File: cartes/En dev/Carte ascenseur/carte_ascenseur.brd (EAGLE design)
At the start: 96.5 x 93.9 mm, 35 parts, among them U1 MCP2551, U2 ADUM1250ARZ, U3 ADUM1400ARWZ, X1 12V Dirty, X2 5V Dirty

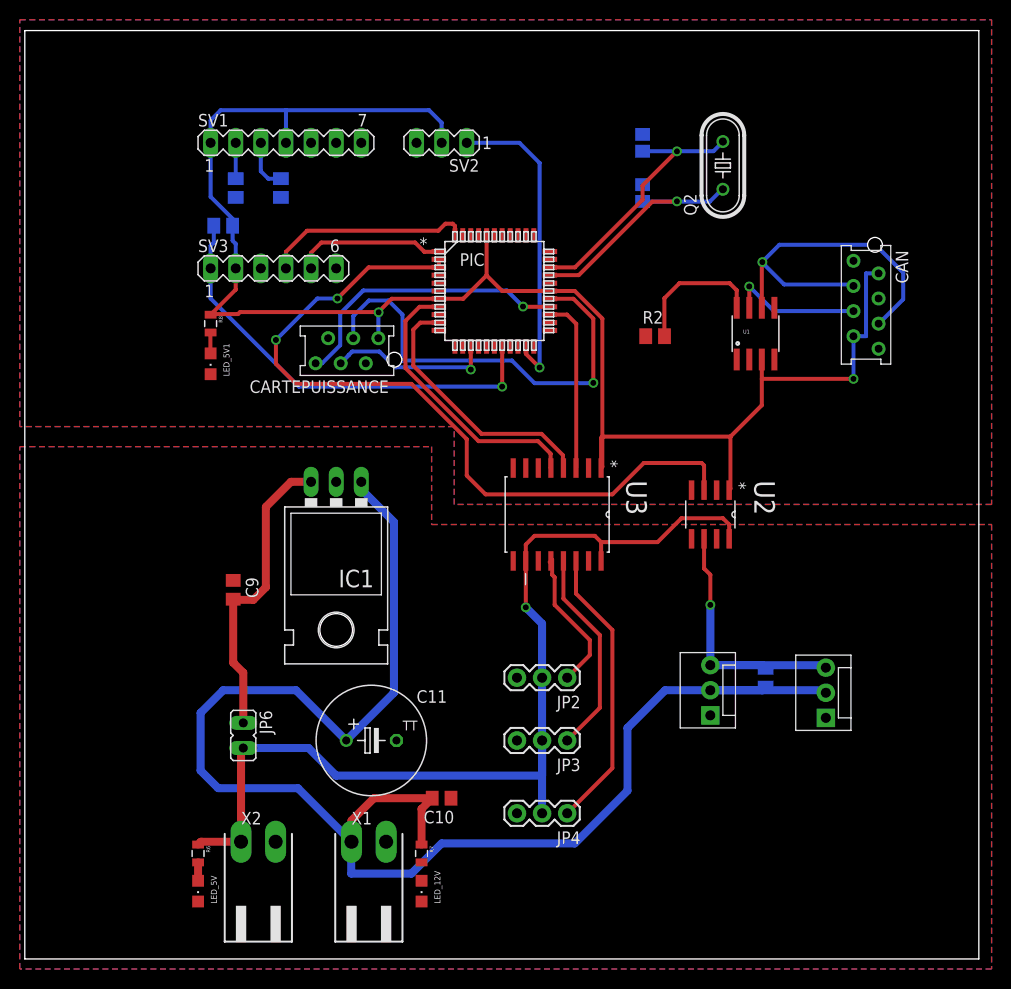
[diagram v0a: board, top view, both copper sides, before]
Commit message: Maj ascenseur
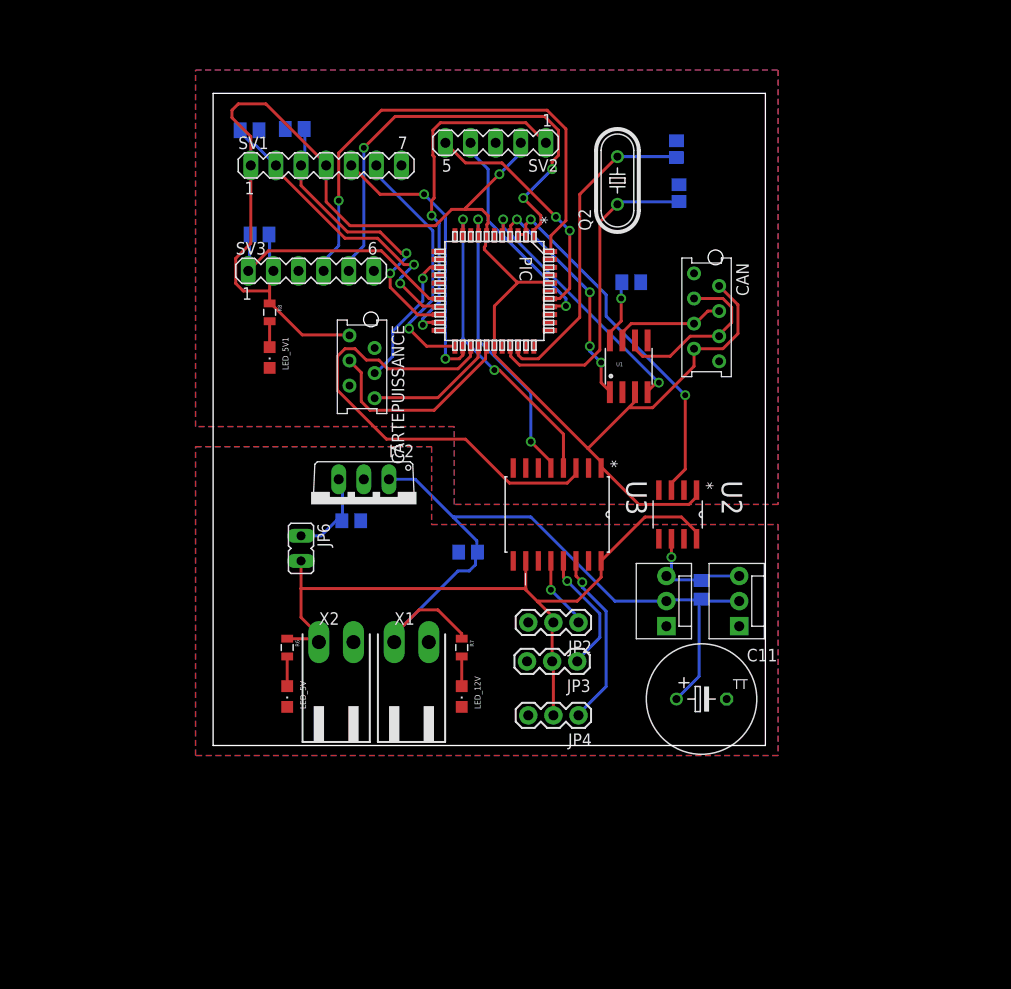
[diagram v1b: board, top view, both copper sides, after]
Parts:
- removed IC1: (no value), SparkFun-PowerIC:TO-220-ALT
- added IC2: 7805TV, linear:TO220V
- SV2: device con-lstb:MA03-1 -> con-lstb:MA05-1
- moved C11 33.7 mm to (65.9, 24.8)
- moved C10 25.0 mm to (42.3, 39.6), flipped to the bottom
- moved R6 22.7 mm to (24.0, 30.0)
- moved X2 21.7 mm to (29.0, 25.3)
- moved LED_5V 21.7 mm to (24.0, 25.0)
- moved R7 21.2 mm to (41.7, 30.0)
- moved X1 20.6 mm to (36.6, 25.3)
- moved LED_12V 20.1 mm to (41.7, 25.0)
- moved JP6 19.8 mm to (25.4, 40.0)
- moved CAN 16.2 mm to (66.4, 67.8)
- moved C9 13.8 mm to (30.5, 42.8), flipped to the bottom, turned to 0 degrees
- moved U1 13.2 mm to (58.5, 58.4)
- moved JP1 12.8 mm to (69.7, 32.1)
- moved R5 11.0 mm to (65.9, 35.8)
- moved Q2 10.8 mm to (57.4, 77.2)
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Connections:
- new net C_S2: PIC.38, SV2.5
- new net C_S3: PIC.37, SV2.4
- net +12V: now also IC2.1; no longer IC1.IN
- net GND2: now also IC2.2; no longer IC1.GND
- net N$6: now also IC2.3; no longer IC1.OUT
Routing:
- net +12V: track 156.2 -> 80.1 mm
- net N$7: track 77.6 -> 37.2 mm
- net PGC: track 15.3 -> 47.8 mm, vias 0 -> 3
- net LANCEUR: track 17.6 -> 48.6 mm
- net PGD: track 21.0 -> 51.2 mm, vias 0 -> 1
- net QEA: track 0.00 -> 28.9 mm, vias 0 -> 2
- net +5V: track 102.7 -> 74.1 mm, vias 1 -> 0
- net FCH: track 3.62 -> 31.0 mm, vias 0 -> 2
- net N$3: track 0.00 -> 26.3 mm, vias 0 -> 2
- net QEB: track 0.00 -> 25.3 mm, vias 0 -> 1
- net C_S2: track 0.00 -> 24.5 mm, vias 0 -> 2
- net FCB: track 5.22 -> 29.6 mm, vias 0 -> 2
- net SENS: track 45.4 -> 21.0 mm
- net N$1: track 0.00 -> 23.3 mm, vias 0 -> 4
- net C_S3: track 0.00 -> 22.2 mm, vias 0 -> 1
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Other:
- board size 96.5 x 93.9 mm -> 55.9 x 66 mm
